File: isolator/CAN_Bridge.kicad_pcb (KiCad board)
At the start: 2 copper layers, 45 parts, among them J1 BOOT1, J2 BOOT0, J3 Power in, J4 JTAG5, J5 USART1, J7 HIGHVOLTAGE CAN, J8 LOWVOLTAGE CAN, SW2 SW_Push, U1 STM32F105RBTx, U2 ISO1050DUB, U4 AZ1117CH-3.3TRG1, U5 MAX3051ESA+, U6 RSH3-1205S, Y2 Crystal_GND24_Small

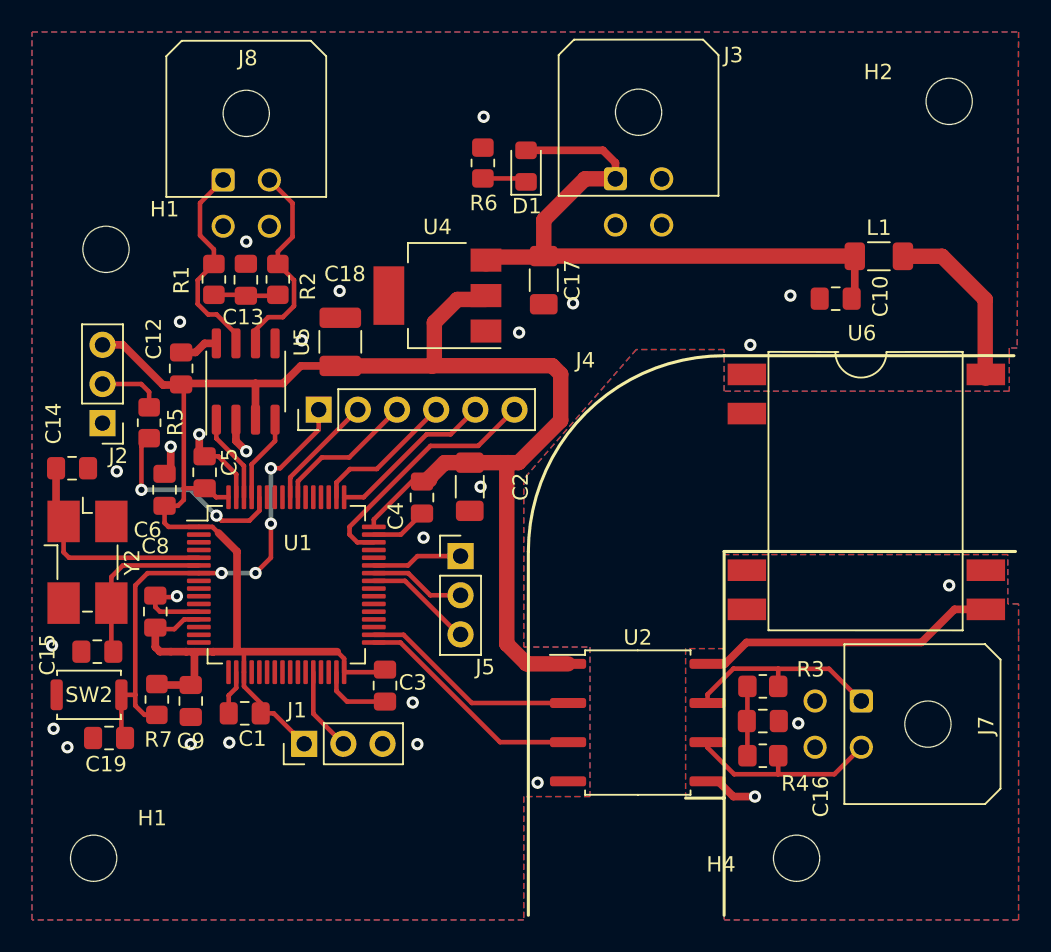
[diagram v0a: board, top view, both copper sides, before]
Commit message: update isolator PCB
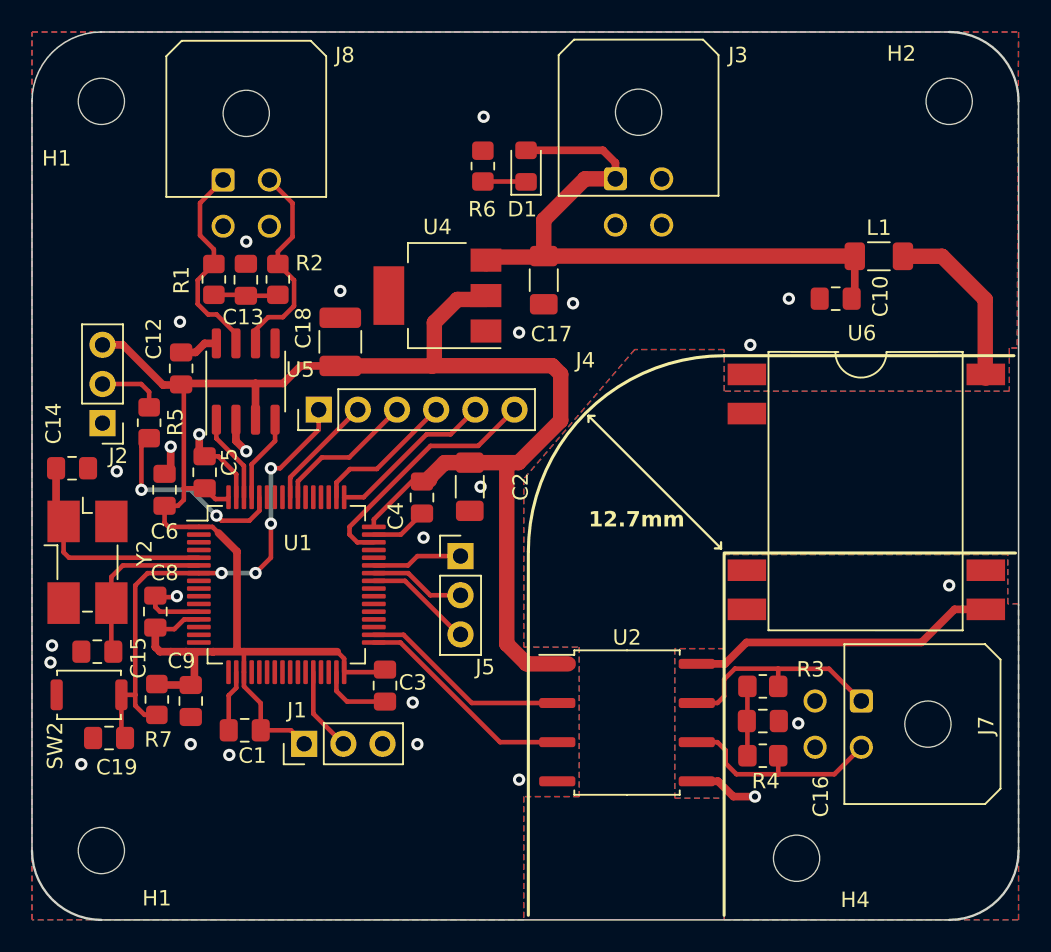
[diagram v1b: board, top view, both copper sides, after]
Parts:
- moved H1 9.60 mm to (135.4, 61.4)
- moved C1 1.10 mm to (144.7, 102.2)
- moved H1 0.71 mm to (135.4, 110.0)
- moved U2 0.70 mm to (169.5, 101.7)
- moved R6 0.20 mm to (160.2, 65.6)
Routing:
- net GND: track 29.8 -> 30.9 mm, vias 24 -> 23
- net HV_CANH: track 13.2 -> 14.2 mm
- net HV_CANL: track 13.0 -> 14.0 mm
- net +3.3V: track 127.8 -> 128.5 mm
- net HV_TXD: track 15.3 -> 14.6 mm
- net HV_RXD: track 14.4 -> 13.7 mm
- net +5P: track 19.5 -> 20.2 mm
- net GND2: track 3.71 -> 4.41 mm
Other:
- board outline added: 64 x 57.6 mm
- board text added: "12.7mm"
